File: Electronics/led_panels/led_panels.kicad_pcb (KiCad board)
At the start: 2 copper layers, 96.5 x 160 mm, 113 parts, among them P1 CONN_2

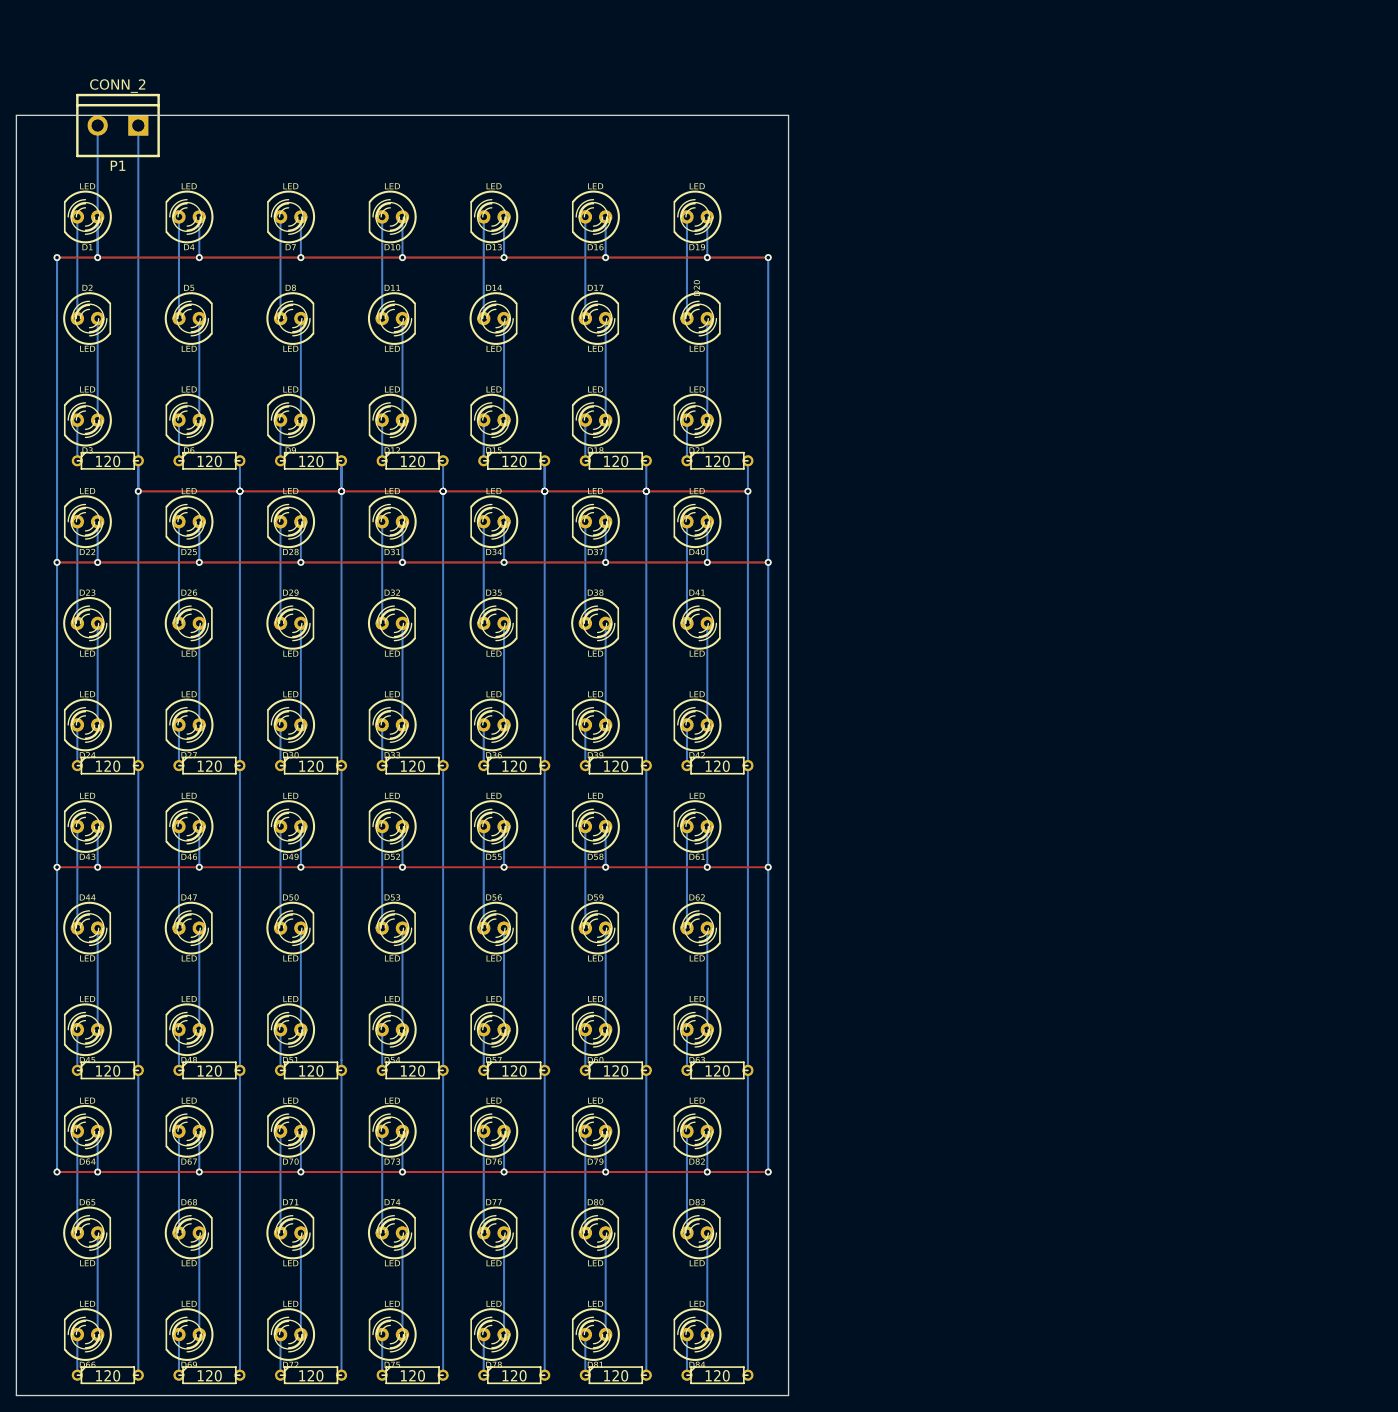
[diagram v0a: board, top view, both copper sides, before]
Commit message: Almost ready for production.
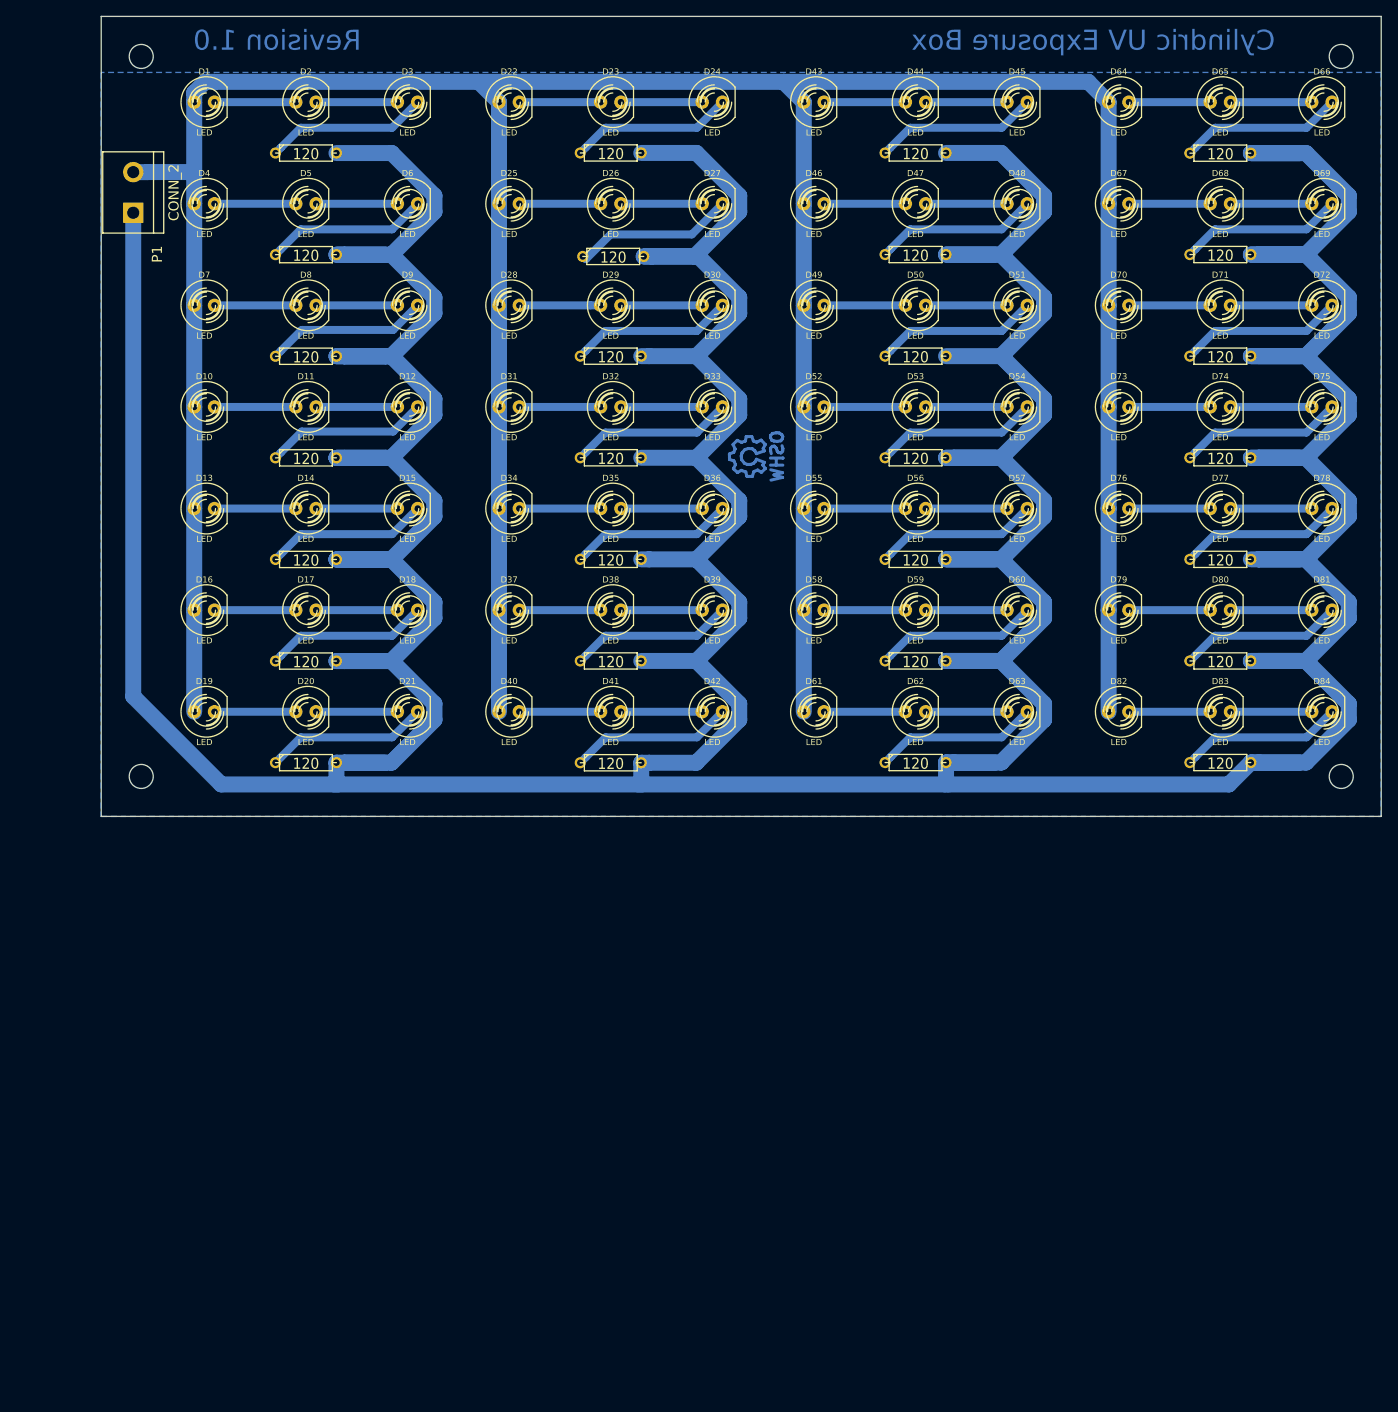
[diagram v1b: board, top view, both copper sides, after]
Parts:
- added MountingHole_3mm: VAL**, Mounting_Holes:MountingHole_3mm, F.Cu at (221.5, 141.1)
- added MountingHole_3mm: VAL**, Mounting_Holes:MountingHole_3mm, F.Cu at (221.5, 51.1)
- added MountingHole_3mm: VAL**, Mounting_Holes:MountingHole_3mm, F.Cu at (71.5, 51.1)
- added MountingHole_3mm: VAL**, Mounting_Holes:MountingHole_3mm, F.Cu at (71.5, 141.1)
- added Symbol_OSHW-Logo_CopperTop: VAL**, Symbols:Symbol_OSHW-Logo_CopperTop, B.Cu at (147.5, 101.1)
- D1, D10, D11, D12, D13, D14, D15, D16, D17, D18, D19, D2, D20, D21, D22, D23, D24, D25, D26, D27, D28, D29, D3, D30, D31, D32, D33, D34, D35, D36, D37, D38, D39, D4, D40, D41, D42, D43, D44, D45, D46, D47, D48, D49, D5, D50, D51, D52, D53, D54, D55, D56, D57, D58, D59, D6, D60, D61, D62, D63, D64, D65, D66, D67, D68, D69, D7, D70, D71, D72, D73, D74, D75, D76, D77, D78, D79, D8, D80, D81, D82, D83, D84, D9: footprint LED-5MM -> LEDs:LED-5MM
- P1: footprint bornier2 -> Connect:bornier2
- R1, R10, R11, R12, R13, R14, R15, R16, R17, R18, R19, R2, R20, R21, R22, R23, R24, R25, R26, R27, R28, R3, R4, R5, R6, R7, R8, R9: footprint R3 -> Discret:R3
- moved D66 218.0 mm to (219.1, 56.8), turned to 0 degrees
- moved R22 206.6 mm to (206.4, 63.1)
- moved D65 200.1 mm to (206.4, 56.8)
- moved D69 200.1 mm to (219.1, 69.5), turned to 0 degrees
- moved R23 188.7 mm to (206.4, 75.8)
- moved D64 182.1 mm to (193.7, 56.8), turned to 0 degrees
- moved D68 182.1 mm to (206.4, 69.5)
- moved D72 182.1 mm to (219.1, 82.2), turned to 0 degrees
- moved R24 170.7 mm to (206.4, 88.5)
- moved D67 164.2 mm to (193.7, 69.5), turned to 0 degrees
- moved D45 164.2 mm to (181.0, 56.8), turned to 0 degrees
- moved D71 164.2 mm to (206.4, 82.2)
- moved D75 164.2 mm to (219.1, 94.9), turned to 0 degrees
- moved R15 152.8 mm to (168.3, 63.1)
- moved R25 152.8 mm to (206.4, 101.2)
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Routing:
- net GND: track 929.6 -> 1302.1 mm, vias 12 -> 0
- net +12V: track 742.9 -> 436.7 mm, vias 36 -> 0
- net Net-(D27-Pad2): track 5.08 -> 20.5 mm
- net Net-(D42-Pad2): track 5.08 -> 20.4 mm
- net Net-(D66-Pad2): track 5.08 -> 20.4 mm
- net Net-(D21-Pad2): track 5.08 -> 20.4 mm
- net Net-(D9-Pad2): track 5.08 -> 20.4 mm
- net Net-(D6-Pad2): track 5.08 -> 20.4 mm
- net Net-(D12-Pad2): track 5.08 -> 20.4 mm
- net Net-(D3-Pad2): track 5.08 -> 20.4 mm
- net Net-(D15-Pad2): track 5.08 -> 20.4 mm
- net Net-(D18-Pad2): track 5.08 -> 20.4 mm
- net Net-(D30-Pad2): track 5.08 -> 20.4 mm
- net Net-(D24-Pad2): track 5.08 -> 20.4 mm
- net Net-(D39-Pad2): track 5.08 -> 20.4 mm
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- added copper zone on B.Cu, net GND
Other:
- board size 96.5 x 160 mm -> 160 x 100 mm
- net class Default: trace_width 0.254 -> 1
- net class Power added: clearance 0.254, trace_width 2, via_dia 0.889, via_drill 0.635
- net class VeroTrack removed
- board text added: "Cylindric UV Exposure Box"
- board text added: "Revision 1.0"
